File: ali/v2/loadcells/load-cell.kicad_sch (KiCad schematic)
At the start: 4 parts

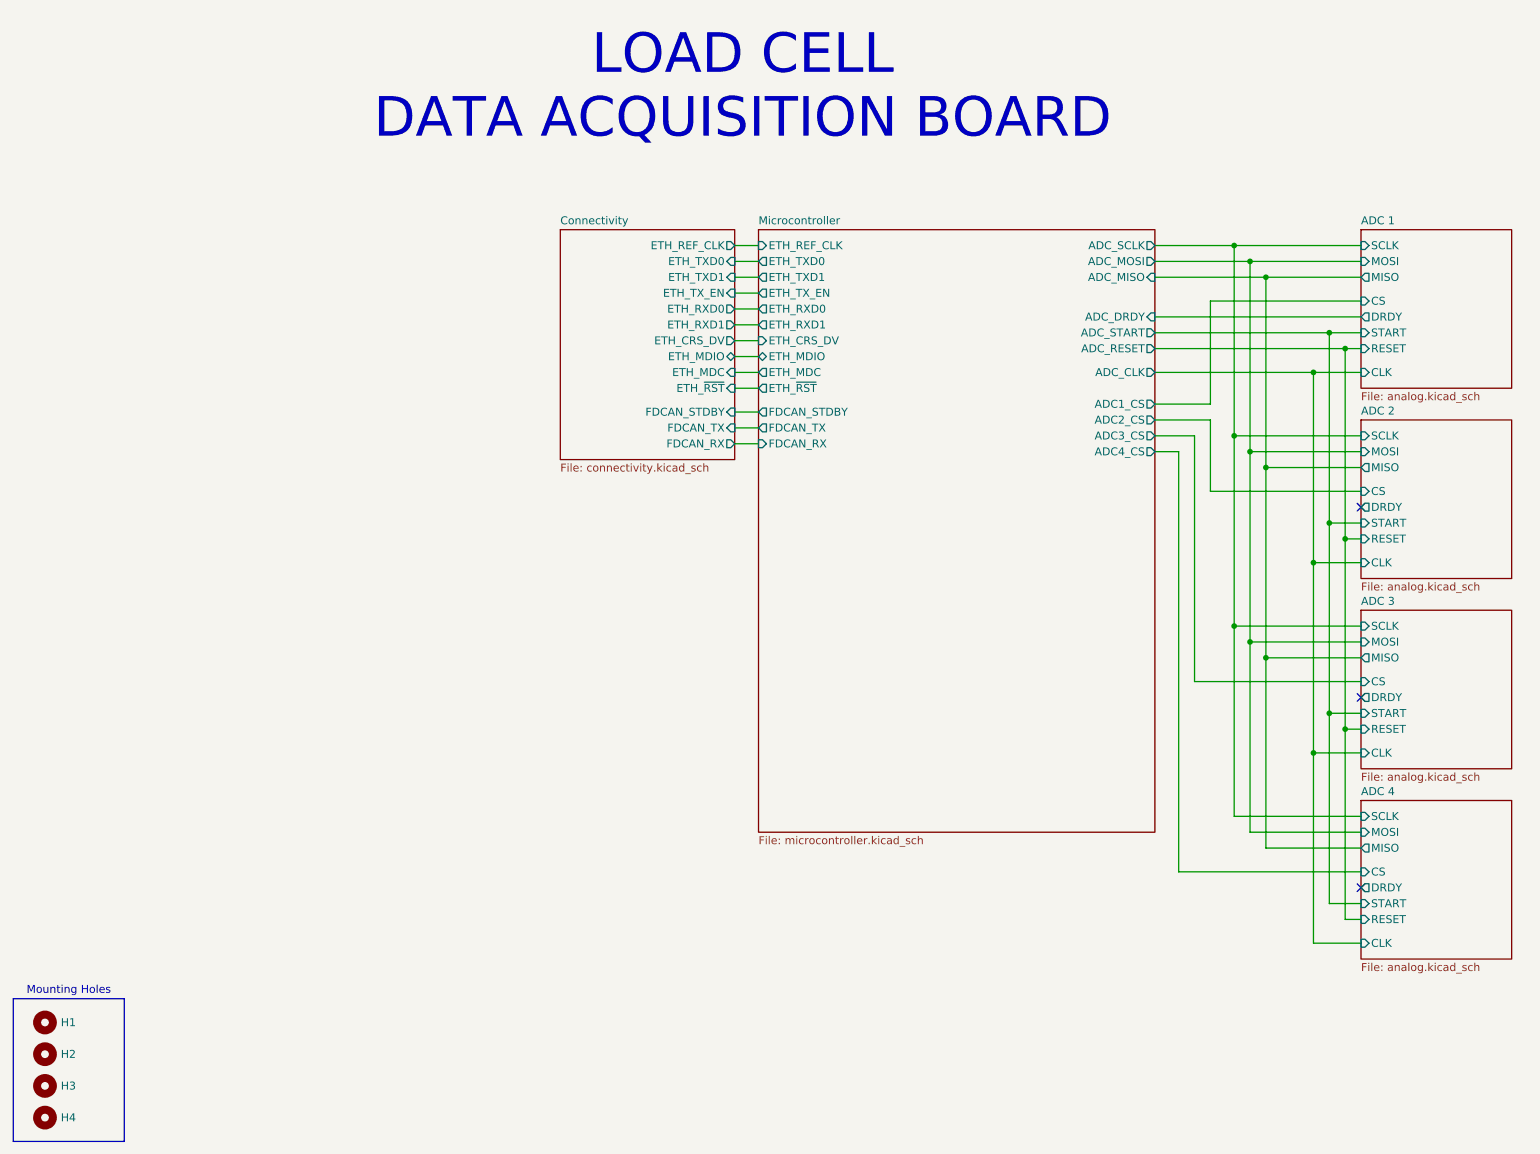
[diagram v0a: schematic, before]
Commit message: Begin prep for second board review
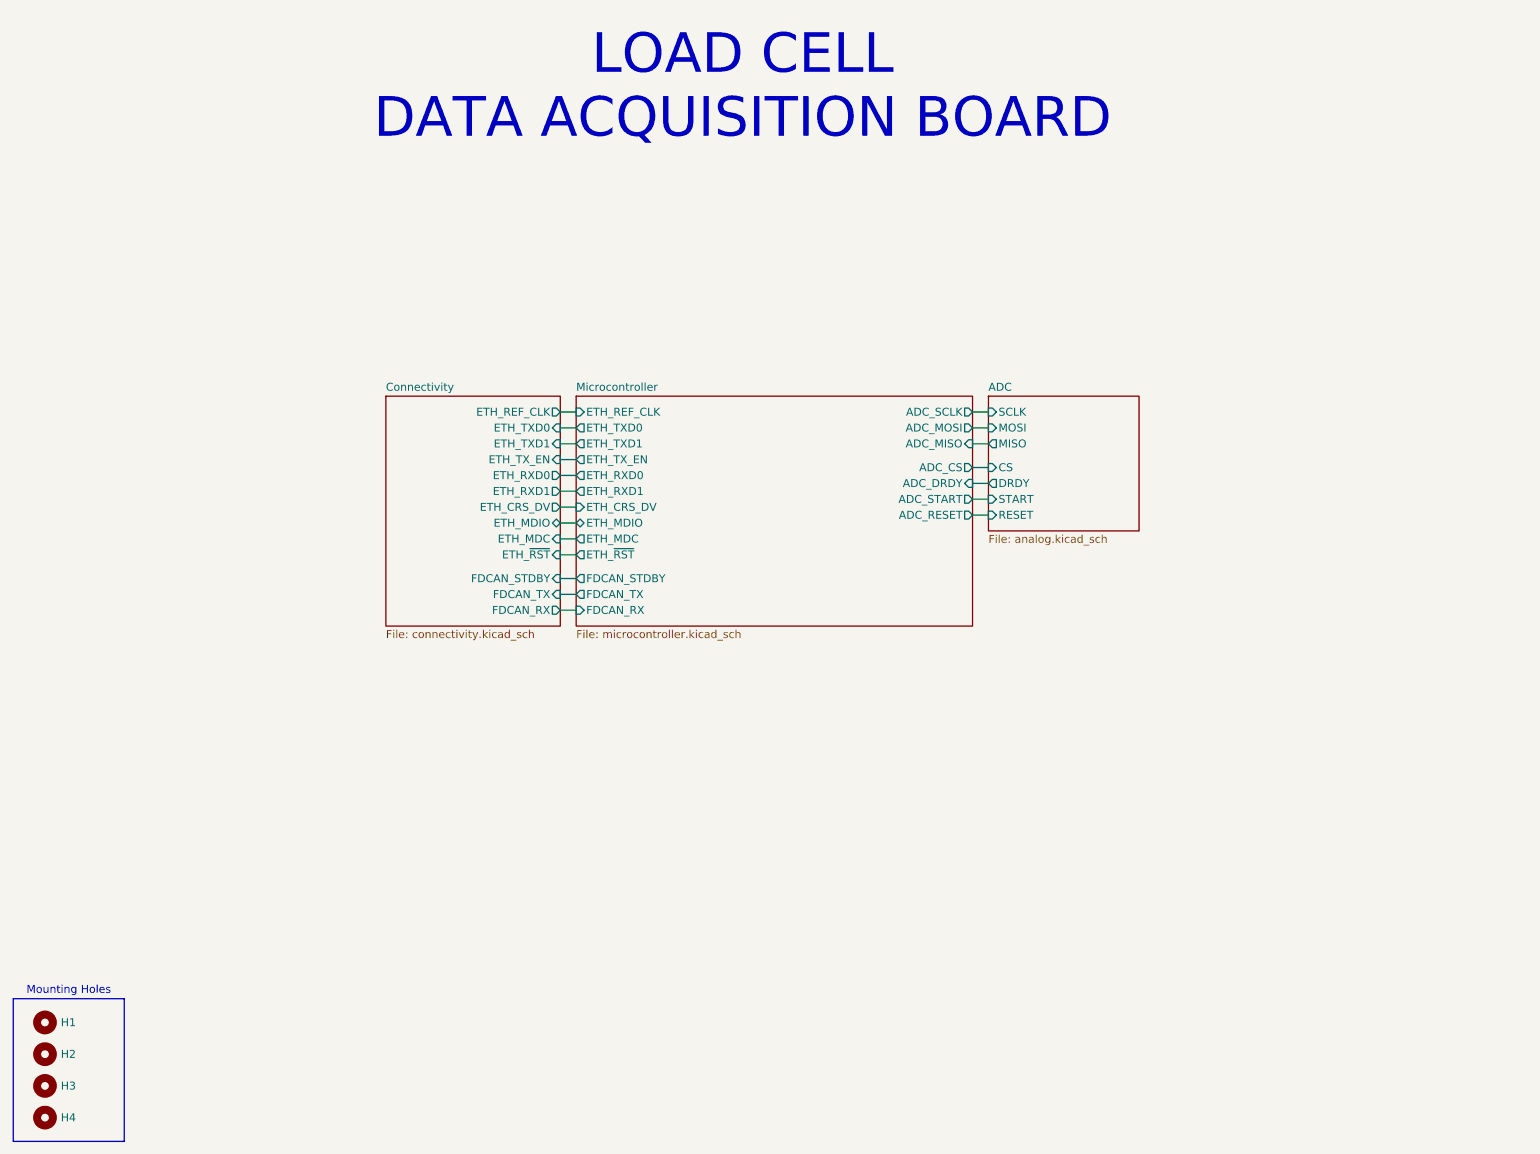
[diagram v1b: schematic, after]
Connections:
- no-connect marks 3 -> 0
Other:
- sheet ADC 1 renamed ADC
- removed sheet ADC 2
- removed sheet ADC 3
- removed sheet ADC 4
- sheet ADC ports: added none; removed CLK
- sheet Microcontroller ports: added ADC_CS; removed ADC1_CS, ADC2_CS, ADC3_CS, ADC4_CS, ADC_CLK
